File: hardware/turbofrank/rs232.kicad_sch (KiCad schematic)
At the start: 10 parts, among them J20 D-SUB 9 Male, U3 MAX232CSE+

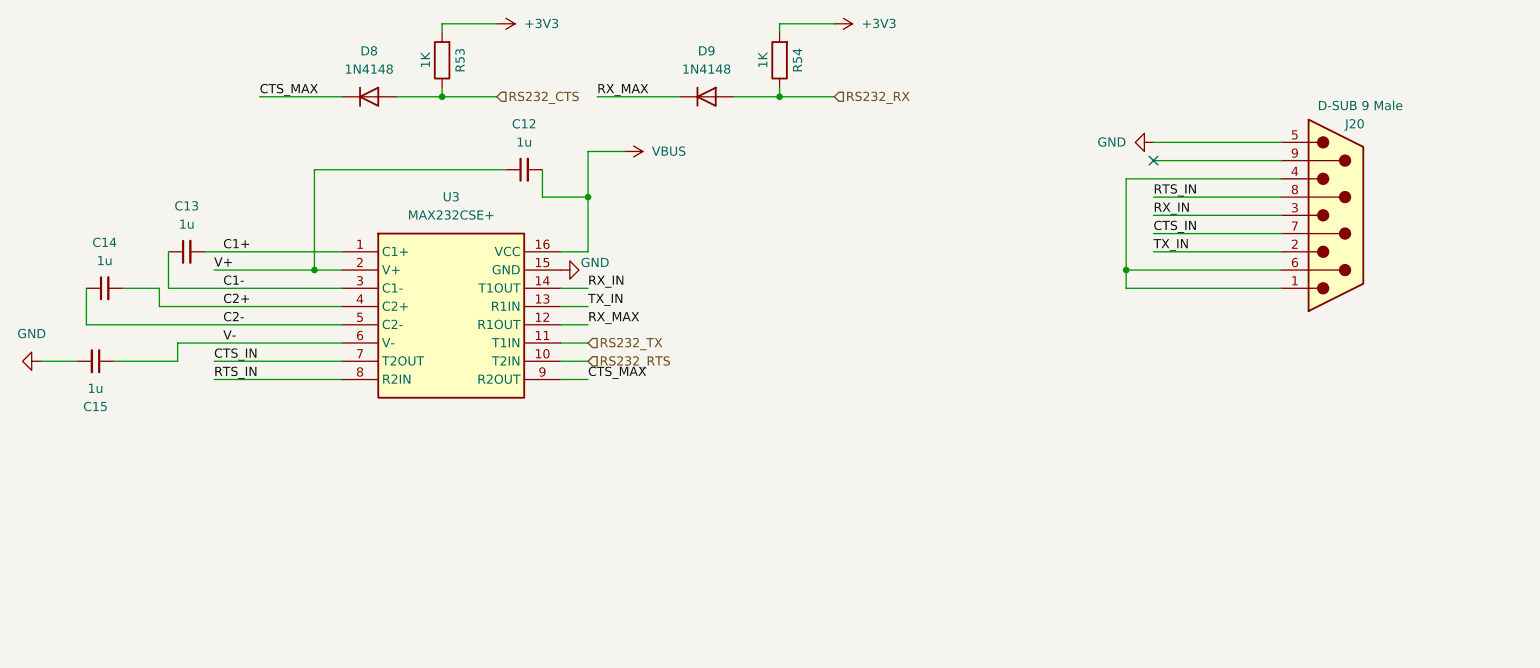
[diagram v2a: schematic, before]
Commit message: TurboFRANK HW 1.05 Release
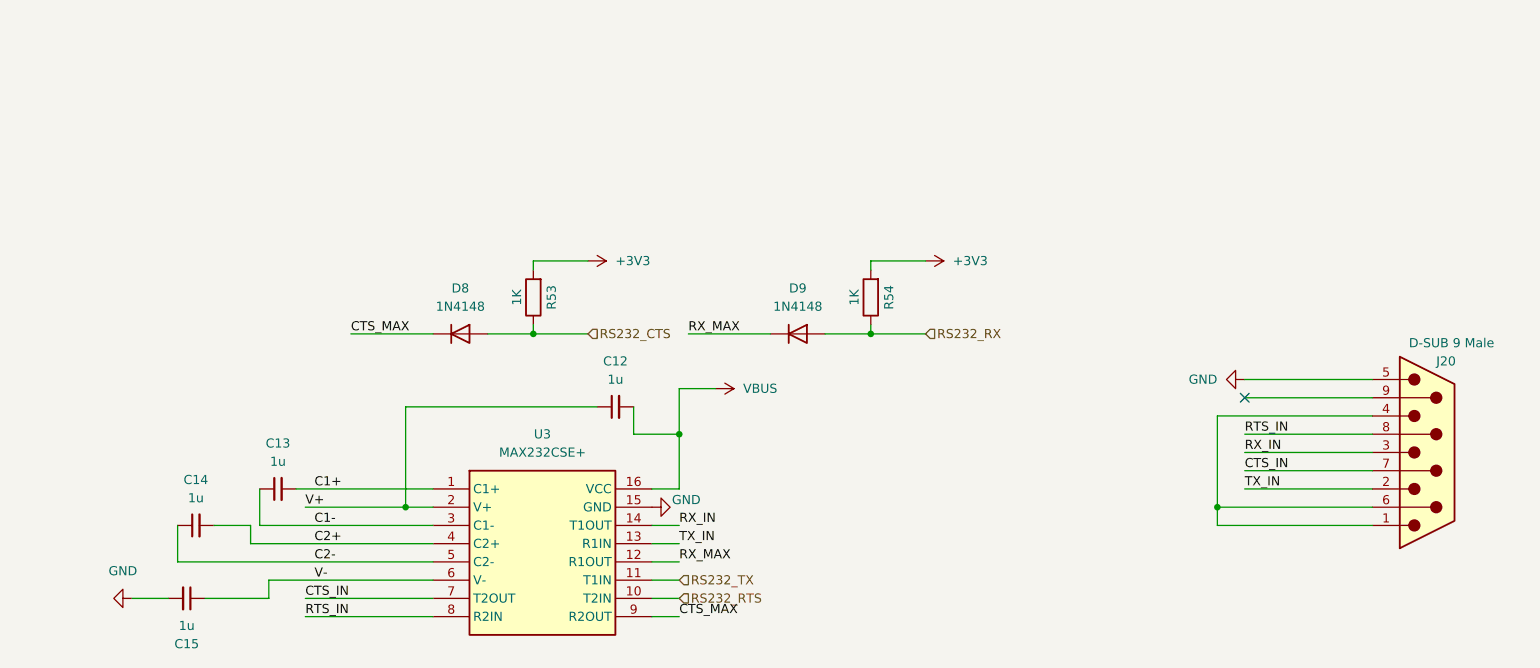
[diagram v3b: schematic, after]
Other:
- moved on the sheet: C12, C13, C14, C15, D8, D9, J20, R53, R54, U3

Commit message: Bugfixes
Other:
- title: TurboFRANK -> ${NAME}
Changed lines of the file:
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@@
 	(paper "A4")
 	(title_block
-		(title "TurboFRANK")
-		(date "2025-04-04")
+		(title "${NAME}")
+		(date "2025-04-20")
 		(rev "${VERSION}")
 		(company "Mikhail Matveev")
